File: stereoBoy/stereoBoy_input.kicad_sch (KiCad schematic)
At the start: 17 parts

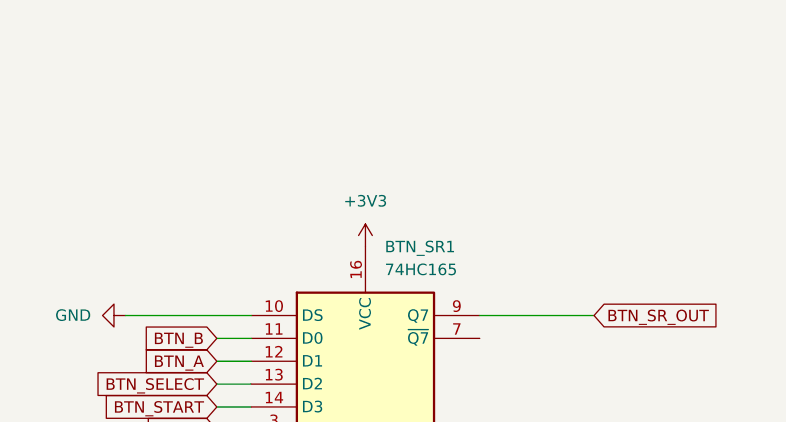
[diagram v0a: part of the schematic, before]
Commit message: yeah
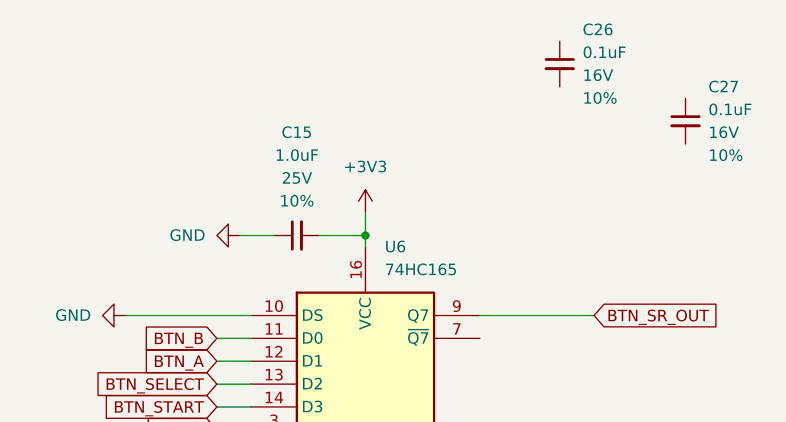
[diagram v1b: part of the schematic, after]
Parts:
- removed BTN_SR1: 74HC165, Package_SO:SOIC-16_3.9x9.9mm_P1.27mm, symbol 74xx:74HC165
- added C15: 1.0uF, SparkFun-Capacitor:C_0805_2012Metric, symbol SparkFun-Capacitor:1.0uF_0805_25V_10%
- added C26, C27: 0.1uF, Capacitor_SMD:C_Elec_5x5.4, symbol SparkFun-Capacitor:0.1uF_0402_16V_10%
- added U6: 74HC165, SparkFun-Semiconductor-Standard:TSSOP-16_4.4x5mm_P0.65mm, symbol 74xx:74HC165
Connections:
- net +3V3: now also C15.2, U6.16 (VCC)
- net BTN_A: now also U6.12 (D1)
- net BTN_B: now also U6.11 (D0)
- net BTN_D: now also U6.6 (D7)
- net BTN_L: now also U6.3 (D4)
- net BTN_R: now also U6.5 (D6)
- net BTN_SELECT: now also U6.13 (D2)
- net BTN_SR_OUT: now also U6.9 (Q7)
- net BTN_START: now also U6.14 (D3)
- net BTN_U: now also U6.4 (D5)
- net GND: now also C15.1, U6.10 (DS), U6.15 (~{CE}), U6.8 (GND)

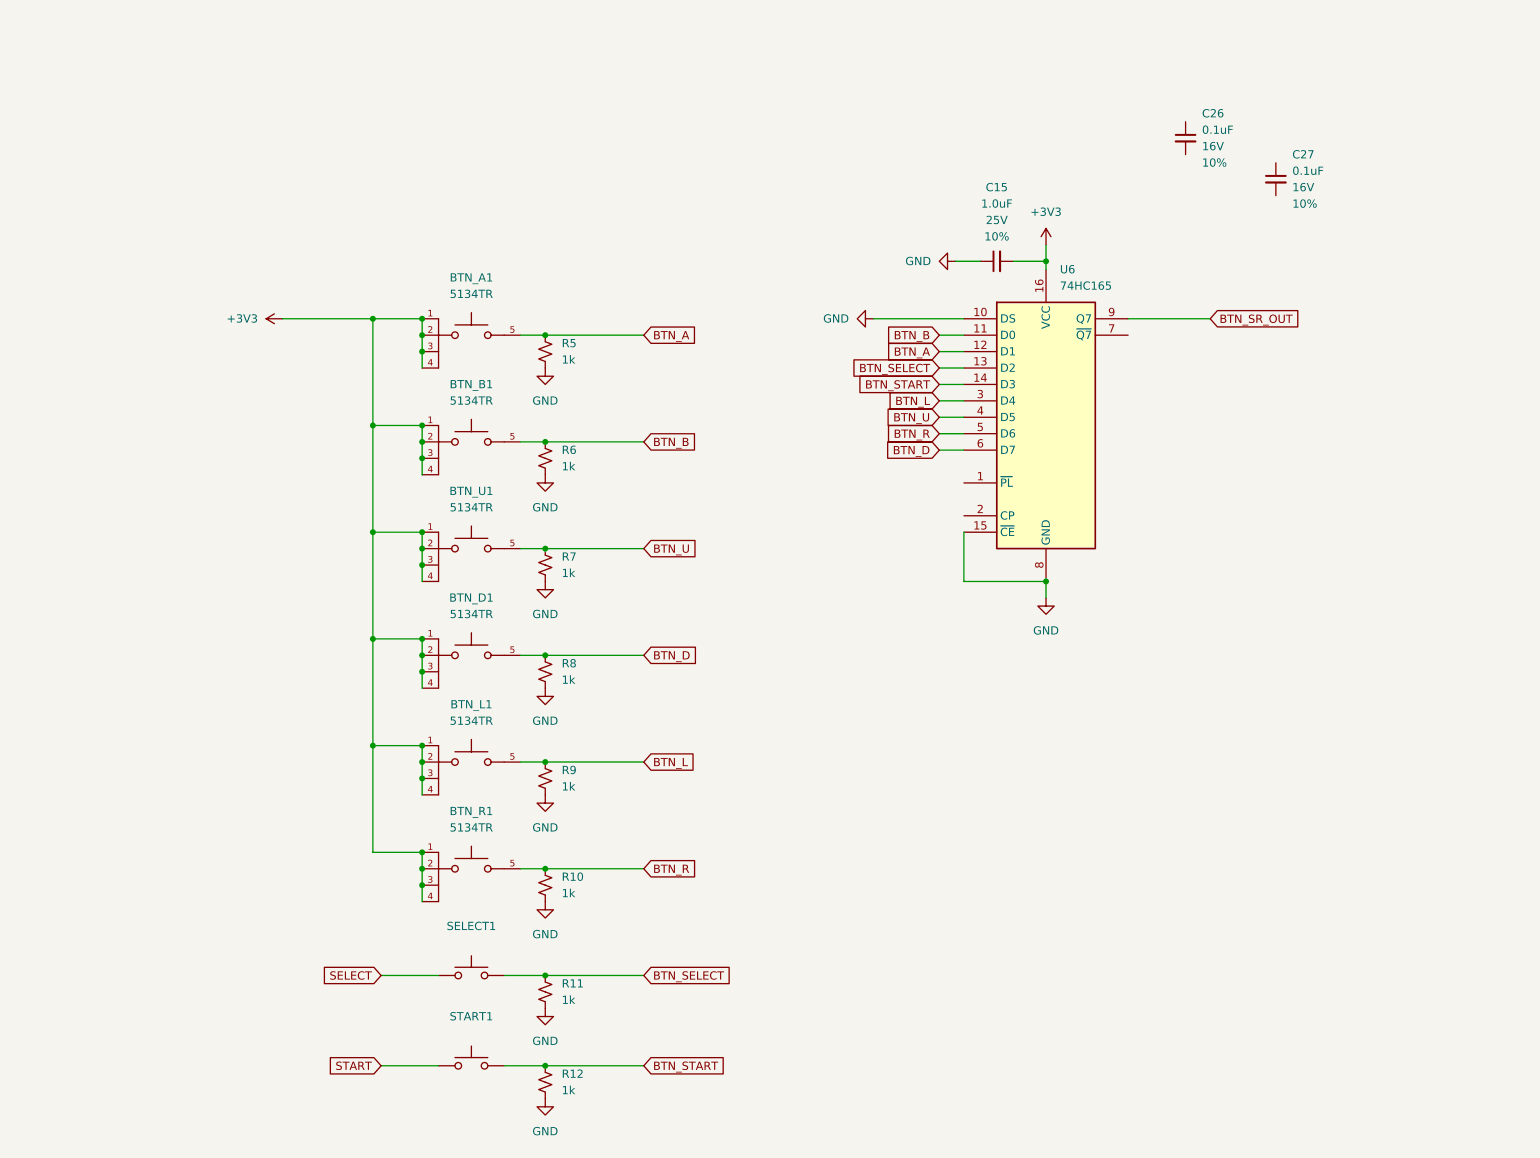
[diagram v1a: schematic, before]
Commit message: yuh
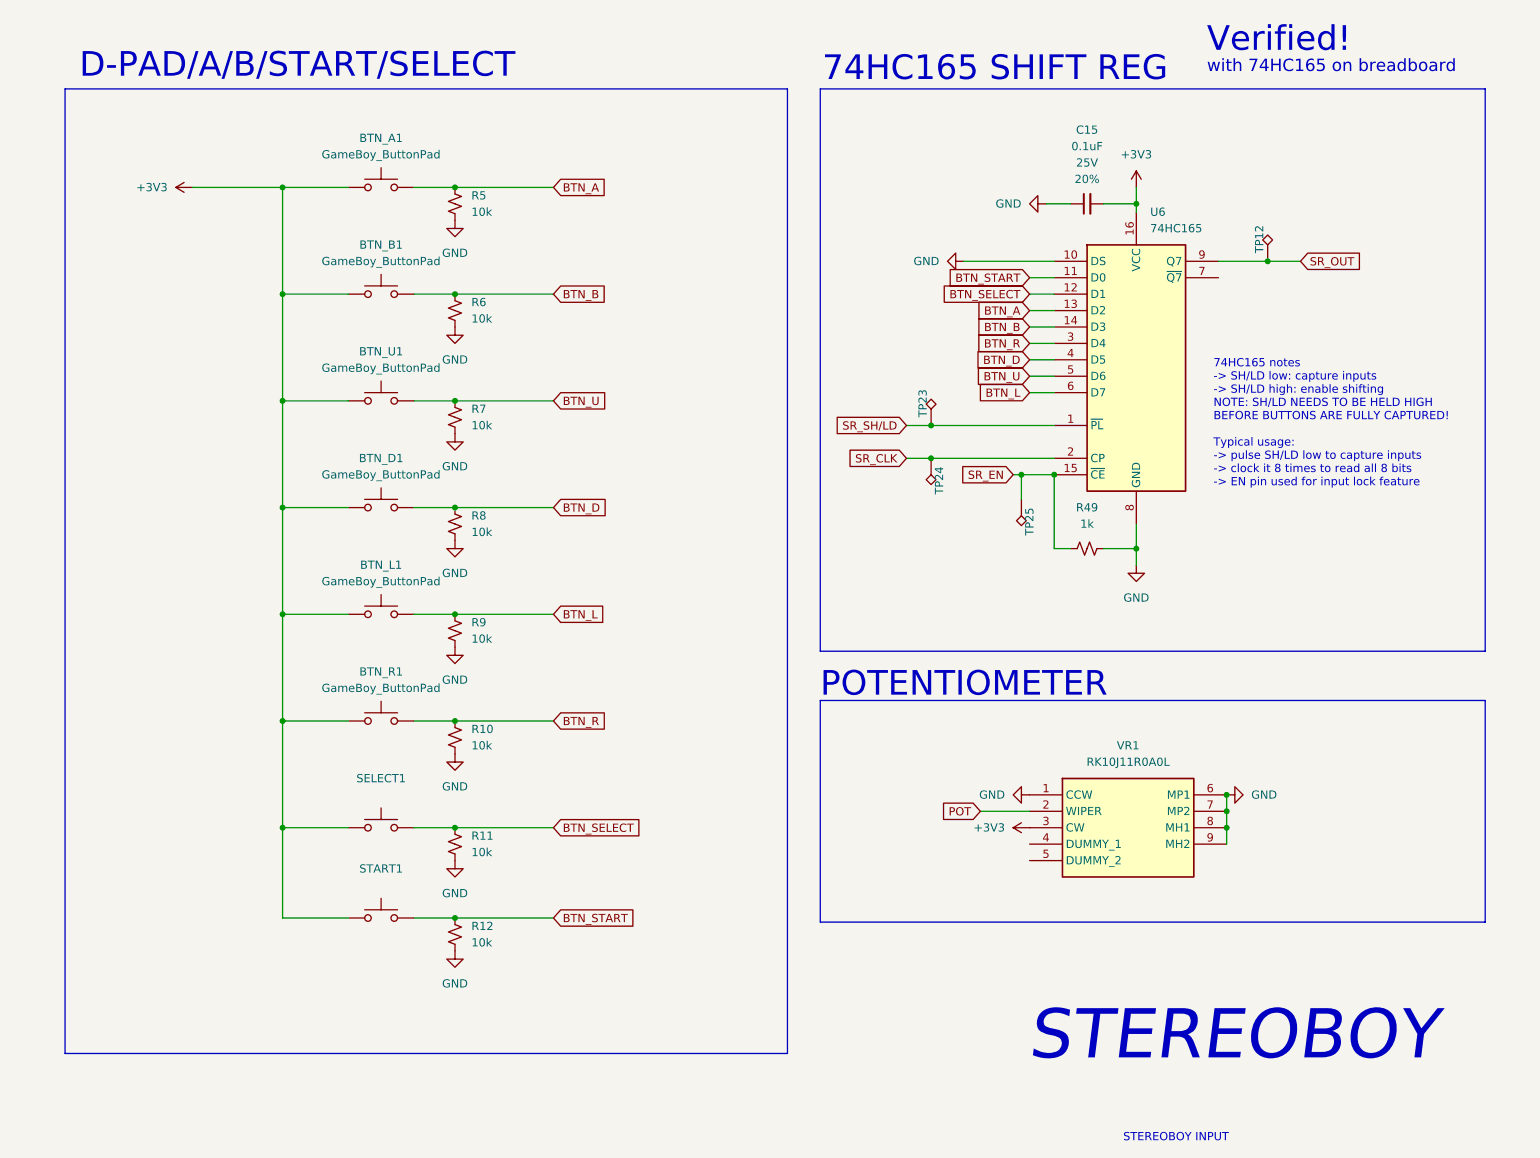
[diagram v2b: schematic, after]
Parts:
- removed BTN_A1, BTN_B1, BTN_D1, BTN_L1, BTN_R1, BTN_U1: 5134TR, SNAP_DOME_SWITCH_7x7:SNAP_DOME_SWITCH_7x7, symbol SNAP_DOME_SWITCH_7x7:5134TR
- removed C15: 1.0uF, SparkFun-Capacitor:C_0805_2012Metric, symbol SparkFun-Capacitor:1.0uF_0805_25V_10%
- removed C26, C27: 0.1uF, Capacitor_SMD:C_Elec_5x5.4, symbol SparkFun-Capacitor:0.1uF_0402_16V_10%
- added BTN_A1, BTN_B1: GameBoy_ButtonPad, GameBoy_ButtonPads:GameBoy_A_B_Pad, symbol SparkFun-Switch:SPST_Push_SMD_RA_5x3mm_h3.6mm
- added BTN_D1, BTN_L1, BTN_R1, BTN_U1: GameBoy_ButtonPad, GameBoy_ButtonPads:GameBoy_DPad, symbol SparkFun-Switch:SPST_Push_SMD_RA_5x3mm_h3.6mm
- added C15: 0.1uF, SparkFun-Capacitor:C_0402_1005Metric, symbol SparkFun-Capacitor:0.1uF_0603_25V_20%
- added R49: 1k, SparkFun-Resistor:R_0402_1005Metric, symbol SparkFun-Resistor:1k_0603
- added TP12, TP23, TP24, TP25: TestPoint_Alt, TestPoint:TestPoint_Pad_D1.0mm, symbol Connector:TestPoint_Alt
- added VR1: RK10J11R0A0L, RK10J11R0A0L:RK10J11R0A0L, symbol RK10J11R0A0L:RK10J11R0A0L
- R10, R11, R12, R5, R6, R7, R8, R9: value 1k -> 10k
- SELECT1, START1: footprint GAMEBOY_PARTS:MGB_BUTTONPAD_SELECTSTART -> GameBoy_ButtonPads:GameBoy_Select_Start
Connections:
- net SELECT is gone; now on net +3V3: SELECT1.1
- net START is gone; now on net +3V3: START1.1
- net +3V3: now also BTN_A1.1, BTN_B1.1, BTN_D1.1, BTN_L1.1, BTN_R1.1, BTN_U1.1, C15.2, VR1.3 (CW)
- net BTN_A: now also U6.13 (D2), BTN_A1.2; no longer U6.12 (D1)
- net BTN_B: now also U6.14 (D3), BTN_B1.2; no longer U6.11 (D0)
- net BTN_D: now also U6.4 (D5), BTN_D1.2; no longer U6.6 (D7)
- net BTN_L: now also U6.6 (D7), BTN_L1.2; no longer U6.3 (D4)
- net BTN_R: now also U6.3 (D4), BTN_R1.2; no longer U6.5 (D6)
- net BTN_SELECT: now also U6.12 (D1); no longer U6.13 (D2)
- net BTN_START: now also U6.11 (D0); no longer U6.14 (D3)
- net BTN_U: now also U6.5 (D6), BTN_U1.2; no longer U6.4 (D5)
- net GND: now also C15.1, R49.2, VR1.1 (CCW), VR1.6 (MP1), VR1.7 (MP2), VR1.8 (MH1), VR1.9 (MH2); no longer U6.15 (~{CE})
- net SR_SH/LD: now reaches U6.1 (~{PL})
- net SR_SH/LD: now also TP23.1
- net SR_CLK: now reaches U6.2 (CP)
- net SR_CLK: now also TP24.1
- net BTN_SR_OUT renamed SR_OUT
- net SR_OUT: now also TP12.1
- new net POT: VR1.2 (WIPER)
- new net SR_EN: R49.1, TP25.1, U6.15 (~{CE})
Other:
- note added: "74HC165 SHIFT REG"
- note added: "74HC165 notes -> SH/LD low: capture inputs -> SH/LD high: enable shifting NOTE: SH/LD NEEDS TO BE HELD HIGH BEFORE BUTTONS ARE FULLY CAPTURED! Typical usage: -> pulse SH/LD low to capture inputs -> clock it 8 times to read all 8 bits -> EN pin used for input lock feature"
- note added: "D-PAD/A/B/START/SELECT"
- note added: "POTENTIOMETER"
- note added: "STEREOBOY"
- note added: "STEREOBOY INPUT"
- note added: "Verified!"
- note added: "with 74HC165 on breadboard"
- moved on the sheet: R10, R11, R12, R5, R6, R7, R8, R9, SELECT1, START1, U6
